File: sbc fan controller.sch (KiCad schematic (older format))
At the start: 24 parts, among them CON1 ISP-6, IC1 LM358, J1 Conn_01x13, J2 Conn_01x02, J4 Conn_01x04, J5 Conn_01x04, J6 Conn_01x03, J9 Conn_Coaxial, Q1 Q_PMOS_GSD, U1 ATTINY13A-SSU, U3 4N25

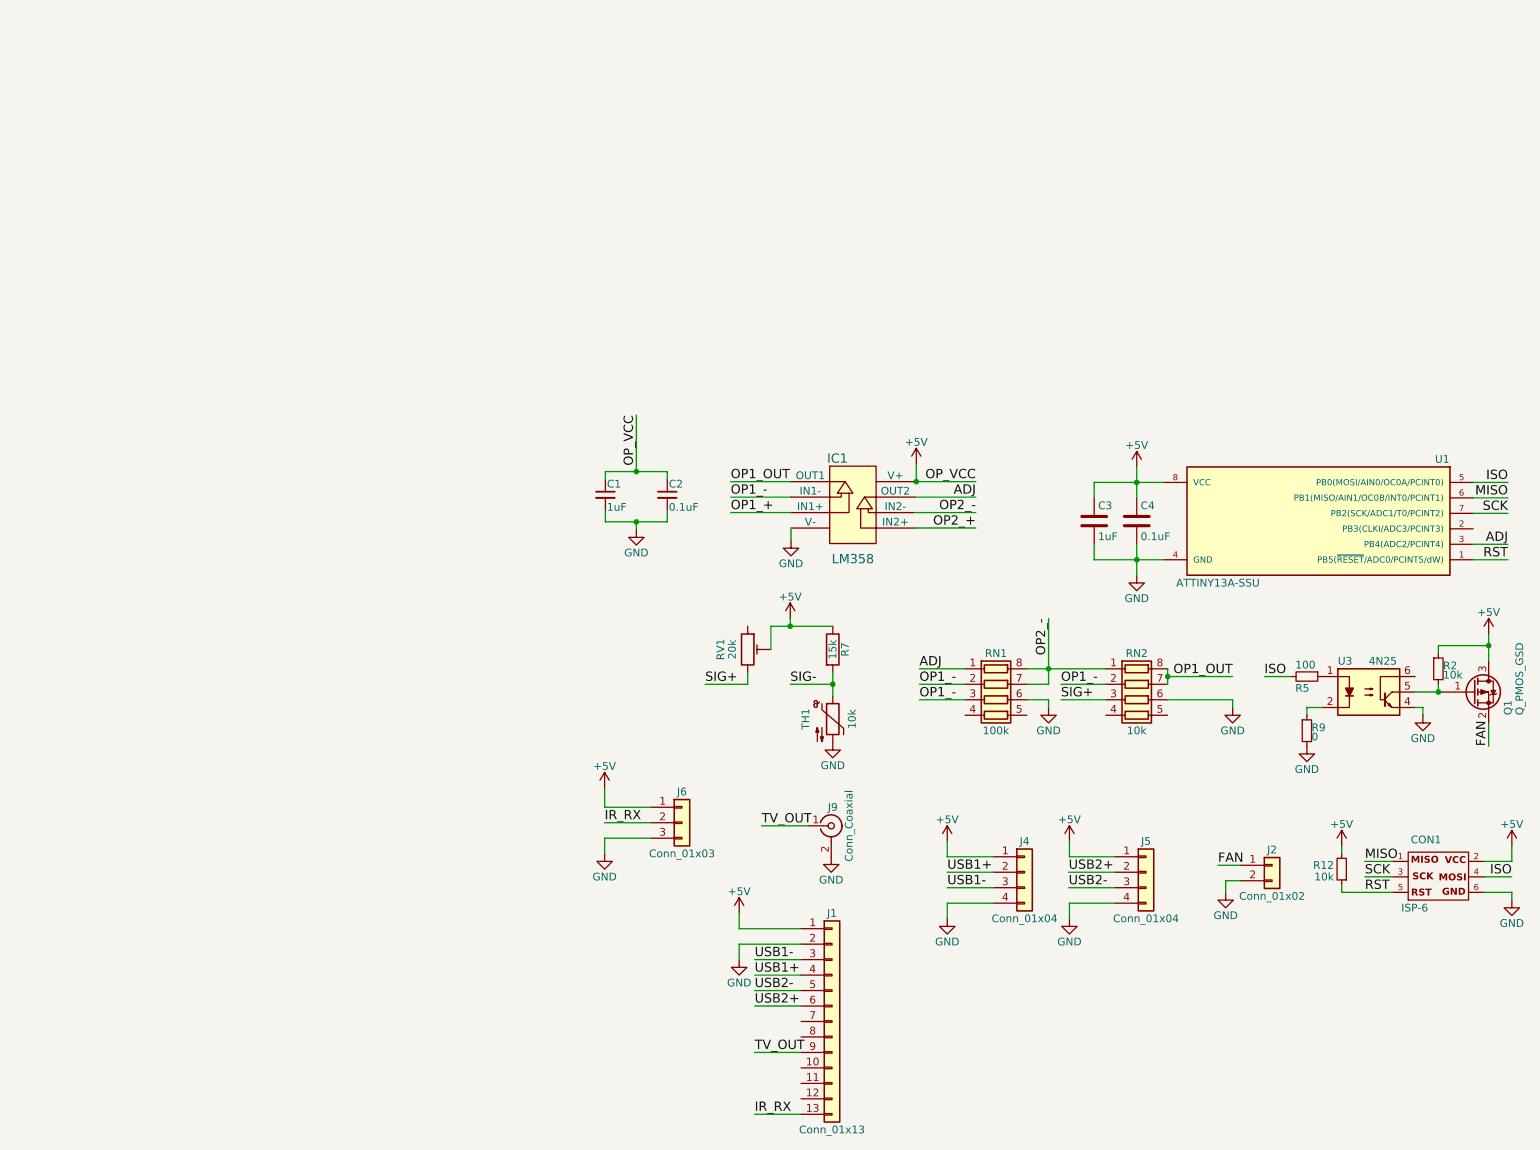
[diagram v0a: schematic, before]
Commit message: Auto stash before merge of "master" and "opi_zero_fan_controller/master"
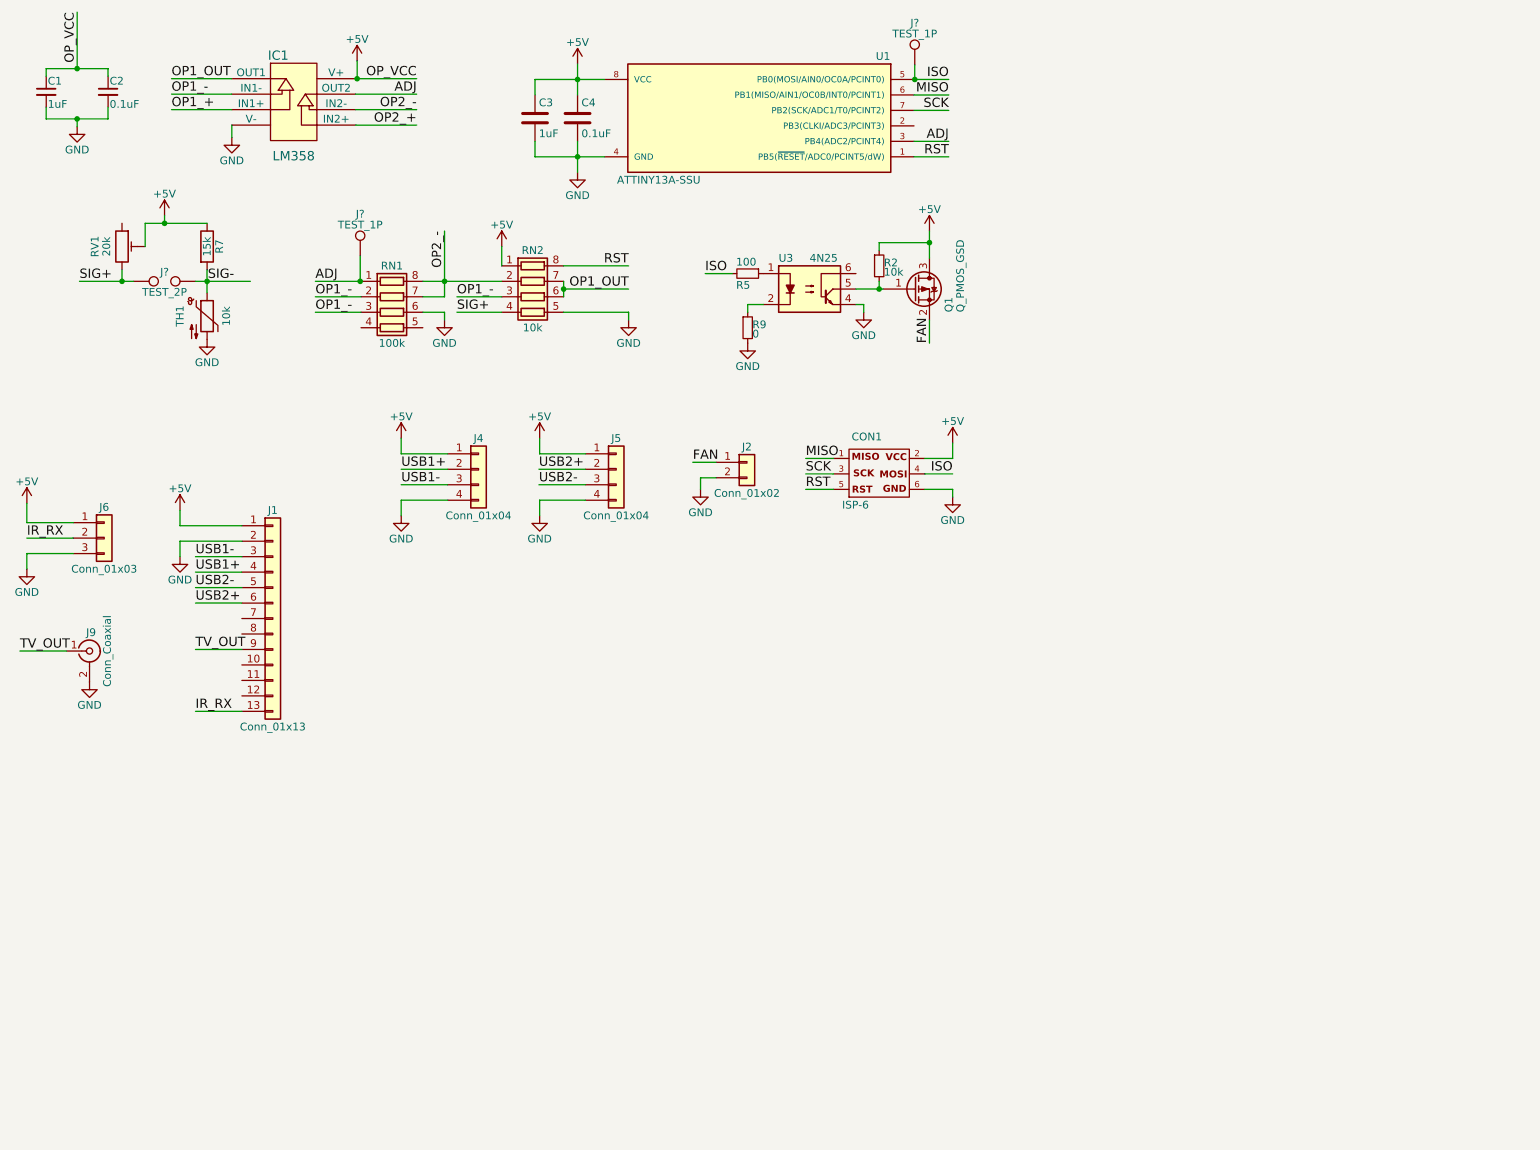
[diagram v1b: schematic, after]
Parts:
- removed R12: 10k, Resistors_SMD:R_0805, symbol R_Small
- added J?: TEST_2P, symbol TEST_2P
- added J? (x2): TEST_1P, symbol TEST_1P
- IC1: footprint (none) -> Housings_SOIC:SOIC-8_3.9x4.9mm_Pitch1.27mm
- RN1, RN2: footprint (none) -> node_nrf:YC164J
- RV1: footprint (none) -> node_nrf:TC33
- U1: footprint Housings_SOIC:SOIC-8_3.9x4.9mm_Pitch1.27mm -> Housings_SOIC:SO-8_5.3x6.2mm_Pitch1.27mm
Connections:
- net +5V: now also RN2.1 (R1.1)
- net ADJ: now also J?.1
- net GND: now also RN2.5 (R4.2); no longer RN2.6 (R3.2)
- net ISO: now also J?.1
- net OP1_-: now also RN2.3 (R3.1); no longer RN2.2 (R2.1)
- net OP1_OUT: now also RN2.6 (R3.2); no longer RN2.8 (R1.2)
- net OP2_-: now also RN2.2 (R2.1); no longer RN2.1 (R1.1)
- net RST: now also RN2.8 (R1.2)
- net SIG+: now also RN2.4 (R4.1), J?.1; no longer RN2.3 (R3.1)
- net SIG-: no longer R7.2, TH1.1
- new net: J?.2, R7.2, TH1.1
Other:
- moved on the sheet: C1, C2, C3, C4, CON1, IC1, J1, J2, J4, J5, J6, J9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
